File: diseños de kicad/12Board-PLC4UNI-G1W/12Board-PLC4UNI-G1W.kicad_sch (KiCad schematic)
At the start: 7 parts, among them J1 Screw_Terminal_01x03, J3 Screw_Terminal_01x03, J4 Screw_Terminal_01x03, J5 Screw_Terminal_01x03, J6 Screw_Terminal_01x03, J7 Screw_Terminal_01x03, J8 Screw_Terminal_01x03

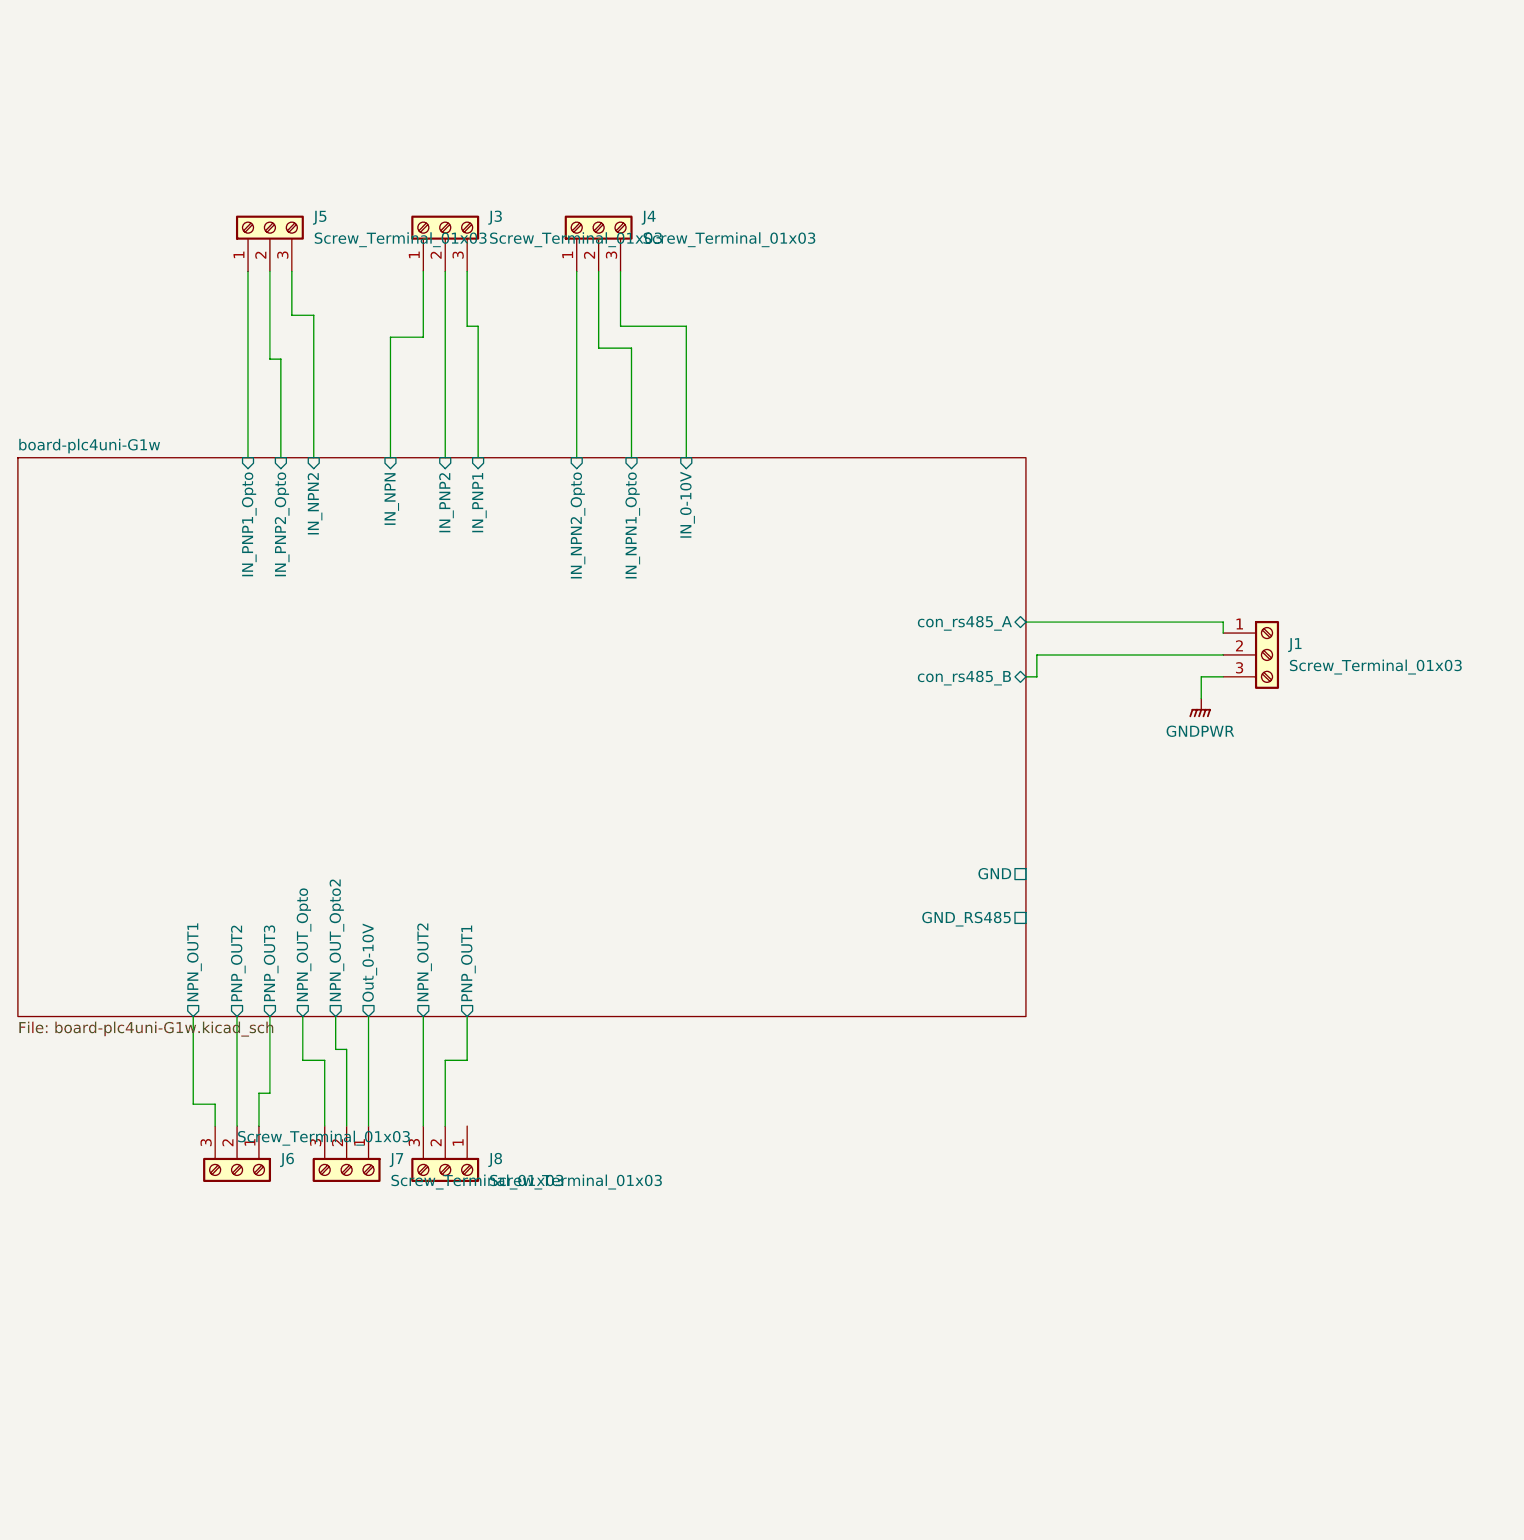
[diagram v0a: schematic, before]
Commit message: actualizacion 47
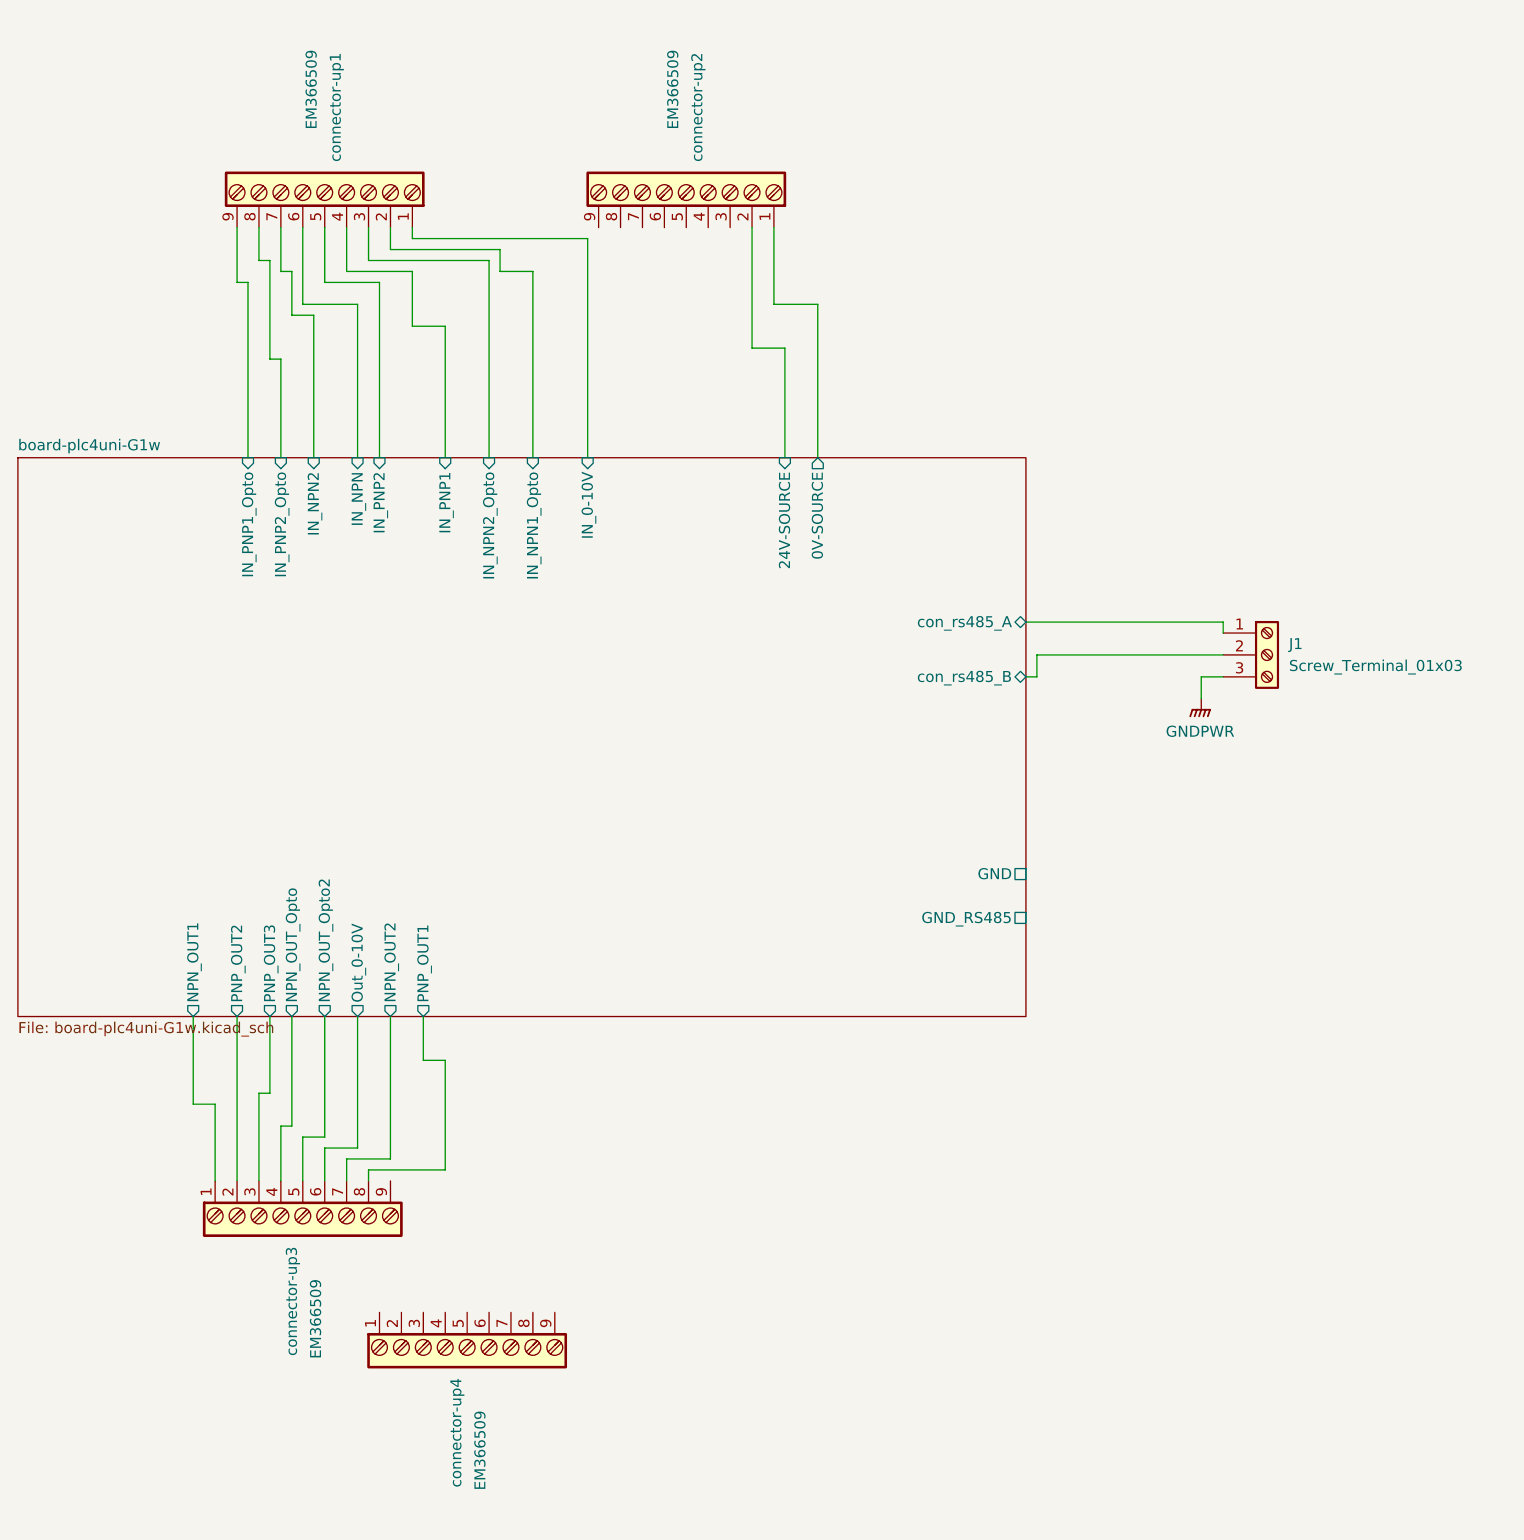
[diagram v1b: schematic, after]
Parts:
- removed J3, J4, J5, J6, J7, J8: Screw_Terminal_01x03, symbol Connector:Screw_Terminal_01x03
- added connector-up1, connector-up2, connector-up3, connector-up4: Screw_Terminal_9_P5.00mm, TerminalBlock_Phoenix:TerminalBlock_Phoenix_PT-1,5-9-5.0-H_1x09_P5.00mm_Horizontal, symbol PCM_SL_Screw_Terminal:Screw_Terminal_9_P5.00mm
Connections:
- net board-plc4uni-G1w/IN_0-10V: now also connector-up1.1
- net board-plc4uni-G1w/IN_NPN: now also connector-up1.6
- net board-plc4uni-G1w/IN_NPN1_Opto: now also connector-up1.2
- net board-plc4uni-G1w/IN_NPN2: now also connector-up1.7
- net board-plc4uni-G1w/IN_NPN2_Opto: now also connector-up1.3
- net board-plc4uni-G1w/IN_PNP1: now also connector-up1.4
- net board-plc4uni-G1w/IN_PNP1_Opto: now also connector-up1.9
- net board-plc4uni-G1w/IN_PNP2: now also connector-up1.5
- net board-plc4uni-G1w/IN_PNP2_Opto: now also connector-up1.8
- net board-plc4uni-G1w/NPN_OUT1: now also connector-up3.1
- net board-plc4uni-G1w/NPN_OUT2: now also connector-up3.7
- net board-plc4uni-G1w/NPN_OUT_Opto: now also connector-up3.4
- net board-plc4uni-G1w/NPN_OUT_Opto2: now also connector-up3.5
- net board-plc4uni-G1w/Out_0-10V: now also connector-up3.6
- net board-plc4uni-G1w/PNP_OUT1: now also connector-up3.8
- net board-plc4uni-G1w/PNP_OUT2: now also connector-up3.2
- net board-plc4uni-G1w/PNP_OUT3: now also connector-up3.3
- new net board-plc4uni-G1w/0V-SOURCE: connector-up2.1
- new net board-plc4uni-G1w/24V-SOURCE: connector-up2.2
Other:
- sheet board-plc4uni-G1w ports: added 0V-SOURCE, 24V-SOURCE; removed none
